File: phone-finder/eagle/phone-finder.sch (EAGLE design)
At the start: 45 parts, among them J1 MICRO USB, J2 PHONE-JACK, K1 RELAY, Q1 DTA114EET1G (2x10K), Q2 2N2222, Q3 2N2222, T1 TRANSFORMER, U1 AP2114H-3.3TRG1, U2 NUF2042XV6T1G, U3 LPC11U35FHI33/501, U4 AMW006, Y1 12Mhz

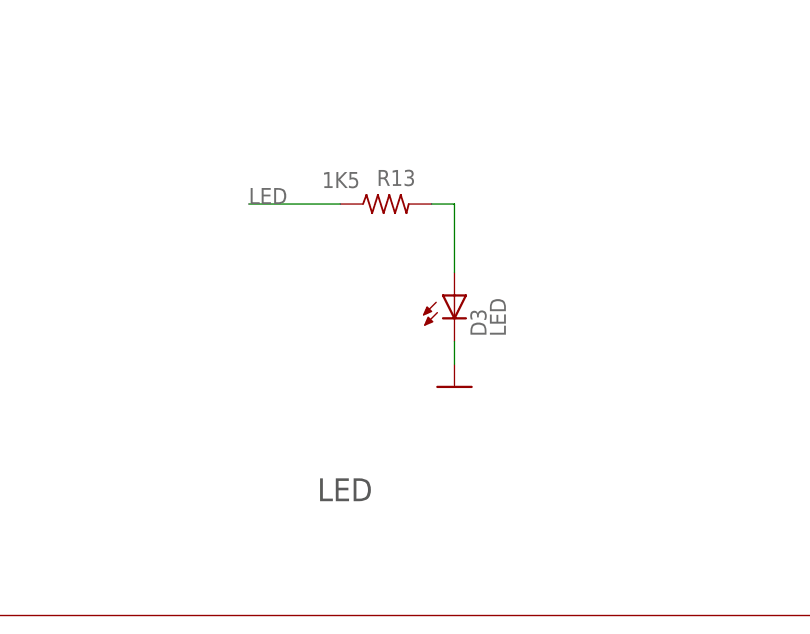
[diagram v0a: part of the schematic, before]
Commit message: Performed final auto routing.
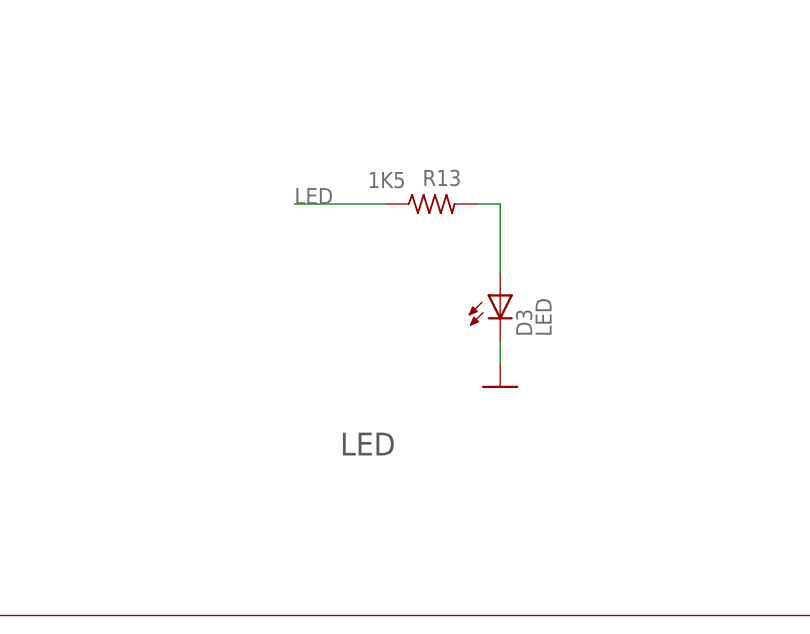
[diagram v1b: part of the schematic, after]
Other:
- moved on the sheet: D3, R13
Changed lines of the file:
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@@
 <wire x1="360.68" y1="73.66" x2="355.6" y2="73.66" width="0.1524" layer="94" style="shortdash"/>
 <text x="287.02" y="81.28" size="2.54" layer="97">PHONE LINE INTERFACE</text>
-<text x="187.96" y="12.7" size="2.54" layer="97">LED</text>
+<text x="190.5" y="17.78" size="2.54" layer="97">LED</text>
 </plain>
 <instances>
@@
 <attribute name="VALUE" x="373.38" y="103.632" size="1.778" layer="96"/>
 </instance>
-<instance part="D3" gate="1" x="203.2" y="35.56"/>
-<instance part="GND10" gate="1" x="203.2" y="25.4"/>
-<instance part="R13" gate="G$1" x="195.58" y="45.72" smashed="yes">
-<attribute name="NAME" x="194.564" y="47.7266" size="1.778" layer="95"/>
-<attribute name="VALUE" x="188.468" y="47.498" size="1.778" layer="96"/>
+<instance part="D3" gate="1" x="208.28" y="35.56"/>
+<instance part="GND10" gate="1" x="208.28" y="25.4"/>
+<instance part="R13" gate="G$1" x="200.66" y="45.72" smashed="yes">
+<attribute name="NAME" x="199.644" y="47.7266" size="1.778" layer="95"/>
+<attribute name="VALUE" x="193.548" y="47.498" size="1.778" layer="96"/>
 </instance>
 </instances>
@@
 <pinref part="D3" gate="1" pin="C"/>
 <pinref part="GND10" gate="1" pin="GND"/>
-<wire x1="203.2" y1="30.48" x2="203.2" y2="27.94" width="0.1524" layer="91"/>
+<wire x1="208.28" y1="30.48" x2="208.28" y2="27.94" width="0.1524" layer="91"/>
 </segment>
 </net>
@@
 <segment>
 <pinref part="R13" gate="G$1" pin="1"/>
-<wire x1="190.5" y1="45.72" x2="180.34" y2="45.72" width="0.1524" layer="91"/>
-<label x="180.34" y="45.72" size="1.778" layer="95"/>
+<wire x1="195.58" y1="45.72" x2="185.42" y2="45.72" width="0.1524" layer="91"/>
+<label x="185.42" y="45.72" size="1.778" layer="95"/>
 </segment>
 </net>
@@
 <pinref part="R13" gate="G$1" pin="2"/>
 <pinref part="D3" gate="1" pin="A"/>
-<wire x1="200.66" y1="45.72" x2="203.2" y2="45.72" width="0.1524" layer="91"/>
-<wire x1="203.2" y1="45.72" x2="203.2" y2="38.1" width="0.1524" layer="91"/>
-</segment>
-</net>
+<wire x1="205.74" y1="45.72" x2="208.28" y2="45.72" width="0.1524" layer="91"/>
+<wire x1="208.28" y1="45.72" x2="208.28" y2="38.1" width="0.1524" layer="91"/>
+</segment>
+</net>
